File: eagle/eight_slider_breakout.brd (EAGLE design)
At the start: 100 x 80 mm, 2 parts, among them CN1 1X4-3.5MM

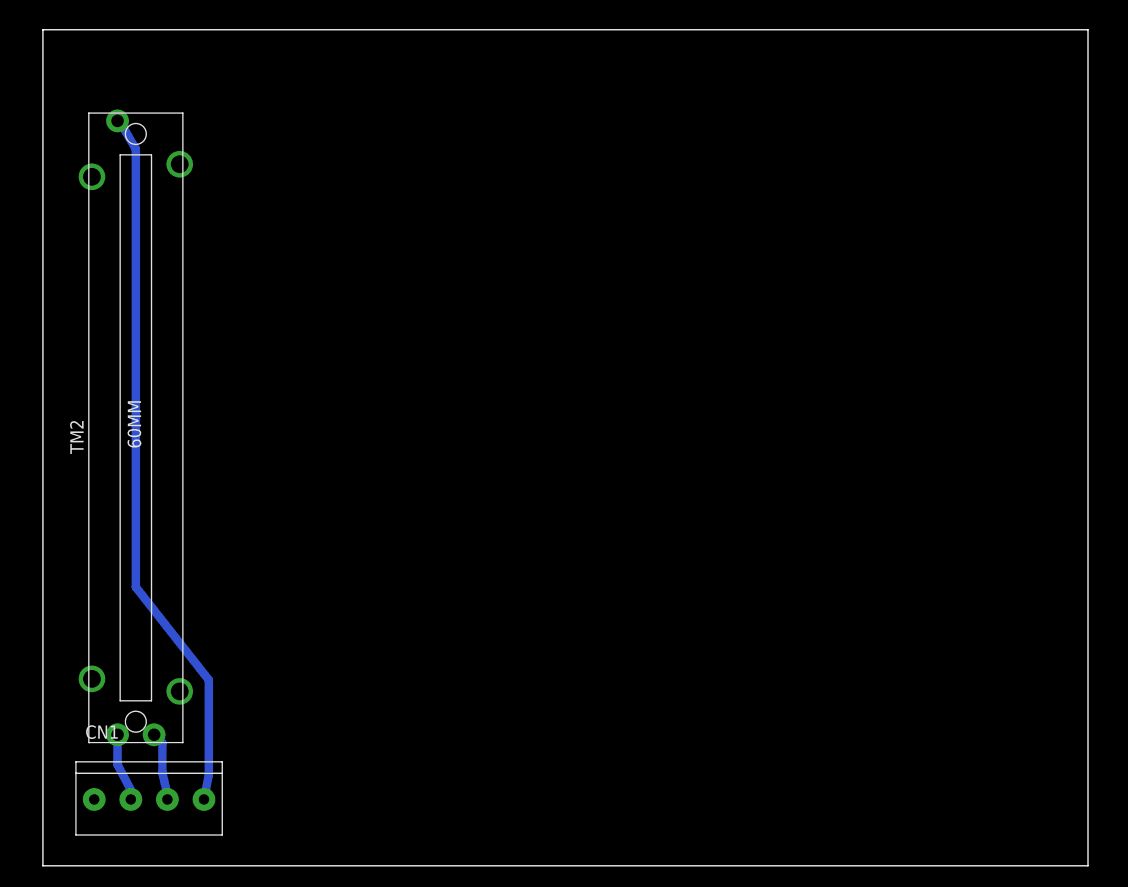
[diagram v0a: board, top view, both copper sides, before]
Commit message: slider board
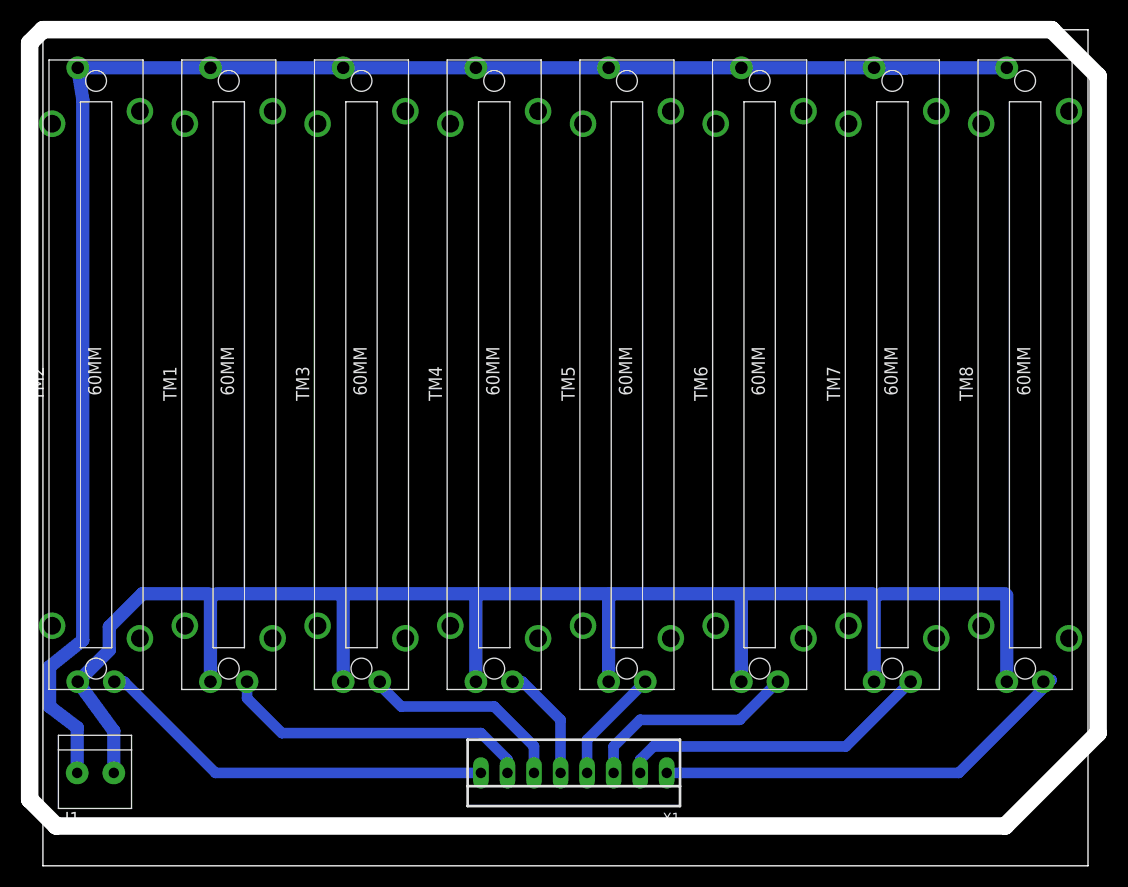
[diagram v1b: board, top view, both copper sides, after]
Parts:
- removed CN1: 1X4-3.5MM, adafruit:1X04-3.5MM
- added J1: 1X2-3.5MM, adafruit:1X2-3.5MM
- added TM1, TM3, TM4, TM5, TM6, TM7, TM8: (no value), stefan-lochbrunner_EAGLE_master_custom libraries_potentiometers_Bourns PTA series_Bourns PTA series:SLIDEPOT-60
- added X1: 22-23-2081, con-molex:22-23-2081
- moved TM2 6.35 mm to (5.08, 47.0)
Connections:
- new net +5V: J1.1, TM1.B, TM2.B, TM3.B, TM4.B, TM5.B, TM6.B, TM7.B, TM8.B
- new net N$3: TM6.WIPER, X1.3
- new net N$4: TM5.WIPER, X1.4
- new net N$5: TM4.WIPER, X1.5
- new net N$6: TM3.WIPER, X1.6
- new net N$7: TM1.WIPER, X1.7
- new net N$8: TM2.WIPER, X1.8
- net GND: now also J1.2, TM1.A, TM3.A, TM4.A, TM5.A, TM6.A, TM7.A, TM8.A; no longer CN1.3
- net N$1: now also TM8.WIPER, X1.1; no longer CN1.1, TM2.B
- net N$2: now also TM7.WIPER, X1.2; no longer CN1.2, TM2.WIPER
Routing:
- net +5V: track 0.00 -> 162.9 mm
- net GND: track 7.78 -> 162.6 mm
- net N$8: track 0.00 -> 38.7 mm
- net N$7: track 0.00 -> 30.2 mm
- net N$1: track 68.5 -> 41.4 mm
- net N$2: track 6.57 -> 30.2 mm
- net N$3: track 0.00 -> 20.8 mm
- net N$6: track 0.00 -> 20.1 mm
- net N$5: track 0.00 -> 11.2 mm
- net N$4: track 0.00 -> 11.0 mm
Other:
- board size 100 x 80 mm -> 102.2 x 80 mm
